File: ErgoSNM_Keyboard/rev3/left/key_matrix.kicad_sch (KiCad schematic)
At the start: 58 parts

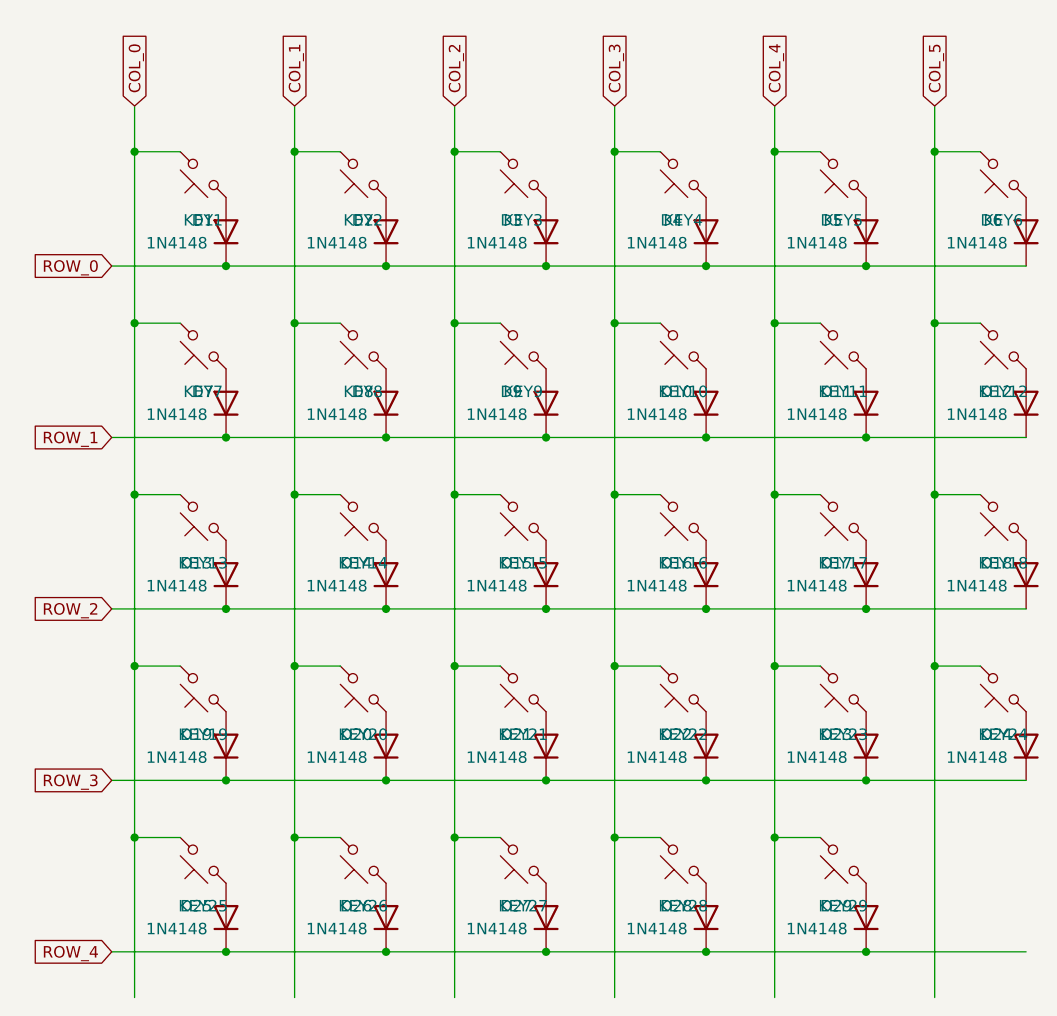
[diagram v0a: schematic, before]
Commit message: Update submodule
Update submodule

Update switch footprint
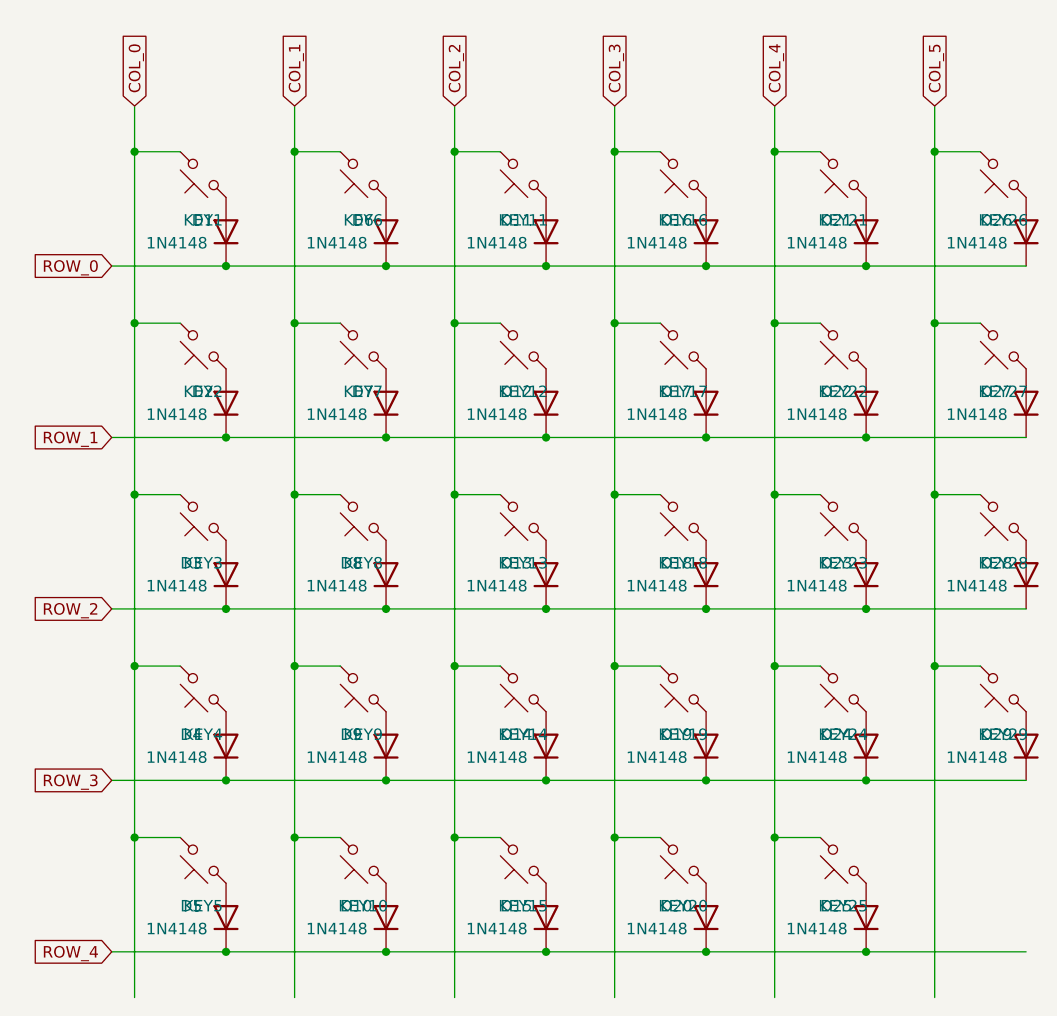
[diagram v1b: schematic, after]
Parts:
- KEY1: footprint key-switches:MX_switch_PTH_hotswap_A -> key-switches:SW_MX_HotSwap_PTH
- KEY10: renamed from KEY26; footprint key-switches:MX_switch_PTH_hotswap_A -> key-switches:SW_MX_HotSwap_PTH
- KEY11: renamed from KEY3; footprint key-switches:MX_switch_PTH_hotswap_A -> key-switches:SW_MX_HotSwap_PTH
- KEY12: renamed from KEY9; footprint key-switches:MX_switch_PTH_hotswap_A -> key-switches:SW_MX_HotSwap_PTH
- KEY13: renamed from KEY15; footprint key-switches:MX_switch_PTH_hotswap_A -> key-switches:SW_MX_HotSwap_PTH
- KEY14: renamed from KEY21; footprint key-switches:MX_switch_PTH_hotswap_A -> key-switches:SW_MX_HotSwap_PTH
- KEY15: renamed from KEY27; footprint key-switches:MX_switch_PTH_hotswap_A -> key-switches:SW_MX_HotSwap_PTH
- KEY16: renamed from KEY4; footprint key-switches:MX_switch_PTH_hotswap_A -> key-switches:SW_MX_HotSwap_PTH
- KEY17: renamed from KEY10; footprint key-switches:MX_switch_PTH_hotswap_A -> key-switches:SW_MX_HotSwap_PTH
- KEY18: renamed from KEY16; footprint key-switches:MX_switch_PTH_hotswap_A -> key-switches:SW_MX_HotSwap_PTH
- KEY19: renamed from KEY22; footprint key-switches:MX_switch_PTH_hotswap_A -> key-switches:SW_MX_HotSwap_PTH
- KEY2: renamed from KEY7; footprint key-switches:MX_switch_PTH_hotswap_A -> key-switches:SW_MX_HotSwap_PTH
- KEY20: renamed from KEY28; footprint key-switches:MX_switch_PTH_hotswap_A -> key-switches:SW_MX_HotSwap_PTH
- KEY21: renamed from KEY5; footprint key-switches:MX_switch_PTH_hotswap_A -> key-switches:SW_MX_HotSwap_PTH
- KEY22: renamed from KEY11; footprint key-switches:MX_switch_PTH_hotswap_A -> key-switches:SW_MX_HotSwap_PTH
- KEY23: renamed from KEY17; footprint key-switches:MX_switch_PTH_hotswap_A -> key-switches:SW_MX_HotSwap_PTH
- KEY24: renamed from KEY23; footprint key-switches:MX_switch_PTH_hotswap_A -> key-switches:SW_MX_HotSwap_PTH
- KEY25: renamed from KEY29; footprint key-switches:MX_switch_PTH_hotswap_A -> key-switches:SW_MX_HotSwap_PTH
- KEY26: renamed from KEY6; footprint key-switches:MX_switch_PTH_hotswap_A -> key-switches:SW_MX_HotSwap_PTH
- KEY27: renamed from KEY12; footprint key-switches:MX_switch_PTH_hotswap_A -> key-switches:SW_MX_HotSwap_PTH
- KEY28: renamed from KEY18; footprint key-switches:MX_switch_PTH_hotswap_A -> key-switches:SW_MX_HotSwap_PTH
- KEY29: renamed from KEY24; footprint key-switches:MX_switch_PTH_hotswap_A -> key-switches:SW_MX_HotSwap_PTH
- KEY3: renamed from KEY13; footprint key-switches:MX_switch_PTH_hotswap_A -> key-switches:SW_MX_HotSwap_PTH
- KEY4: renamed from KEY19; footprint key-switches:MX_switch_PTH_hotswap_A -> key-switches:SW_MX_HotSwap_PTH
- KEY5: renamed from KEY25; footprint key-switches:MX_switch_PTH_hotswap_A -> key-switches:SW_MX_HotSwap_PTH
- KEY6: renamed from KEY2; footprint key-switches:MX_switch_PTH_hotswap_A -> key-switches:SW_MX_HotSwap_PTH
- KEY7: renamed from KEY8; footprint key-switches:MX_switch_PTH_hotswap_A -> key-switches:SW_MX_HotSwap_PTH
- KEY8: renamed from KEY14; footprint key-switches:MX_switch_PTH_hotswap_A -> key-switches:SW_MX_HotSwap_PTH
- KEY9: renamed from KEY20; footprint key-switches:MX_switch_PTH_hotswap_A -> key-switches:SW_MX_HotSwap_PTH
- renumbered D26 to D10, D3 to D11, D9 to D12, D15 to D13, D21 to D14, D27 to D15, D4 to D16, D10 to D17, D16 to D18, D22 to D19, D7 to D2, D28 to D20, D5 to D21, D11 to D22, D17 to D23, D23 to D24, D29 to D25, D6 to D26, D12 to D27, D18 to D28, D24 to D29, D13 to D3, D19 to D4, D25 to D5, D2 to D6, D8 to D7, D14 to D8, D20 to D9
